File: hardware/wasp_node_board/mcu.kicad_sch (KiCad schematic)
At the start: 33 parts, among them J6 TC2030, SW2 C&K KMR231NG LFS, U1 STM32H723ZGTx, U3 APS6404L-3SQRx-SN, Y2 ASE-25.000MHZ-L-K-T

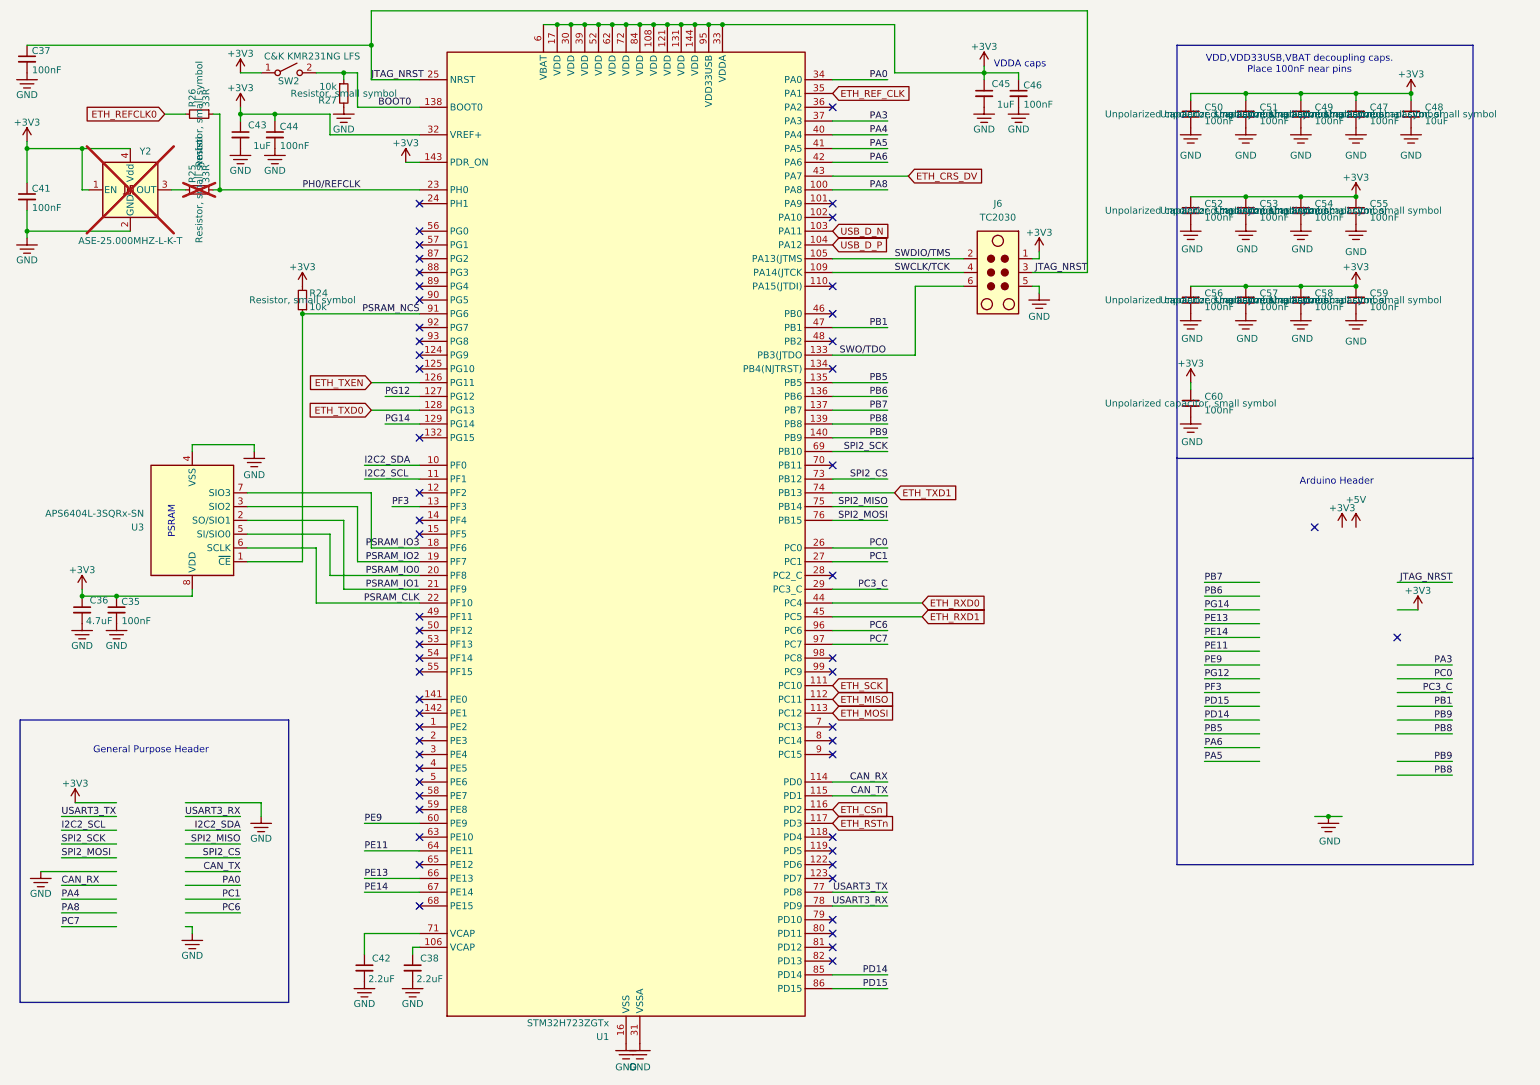
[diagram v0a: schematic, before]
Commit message: V1 layout done
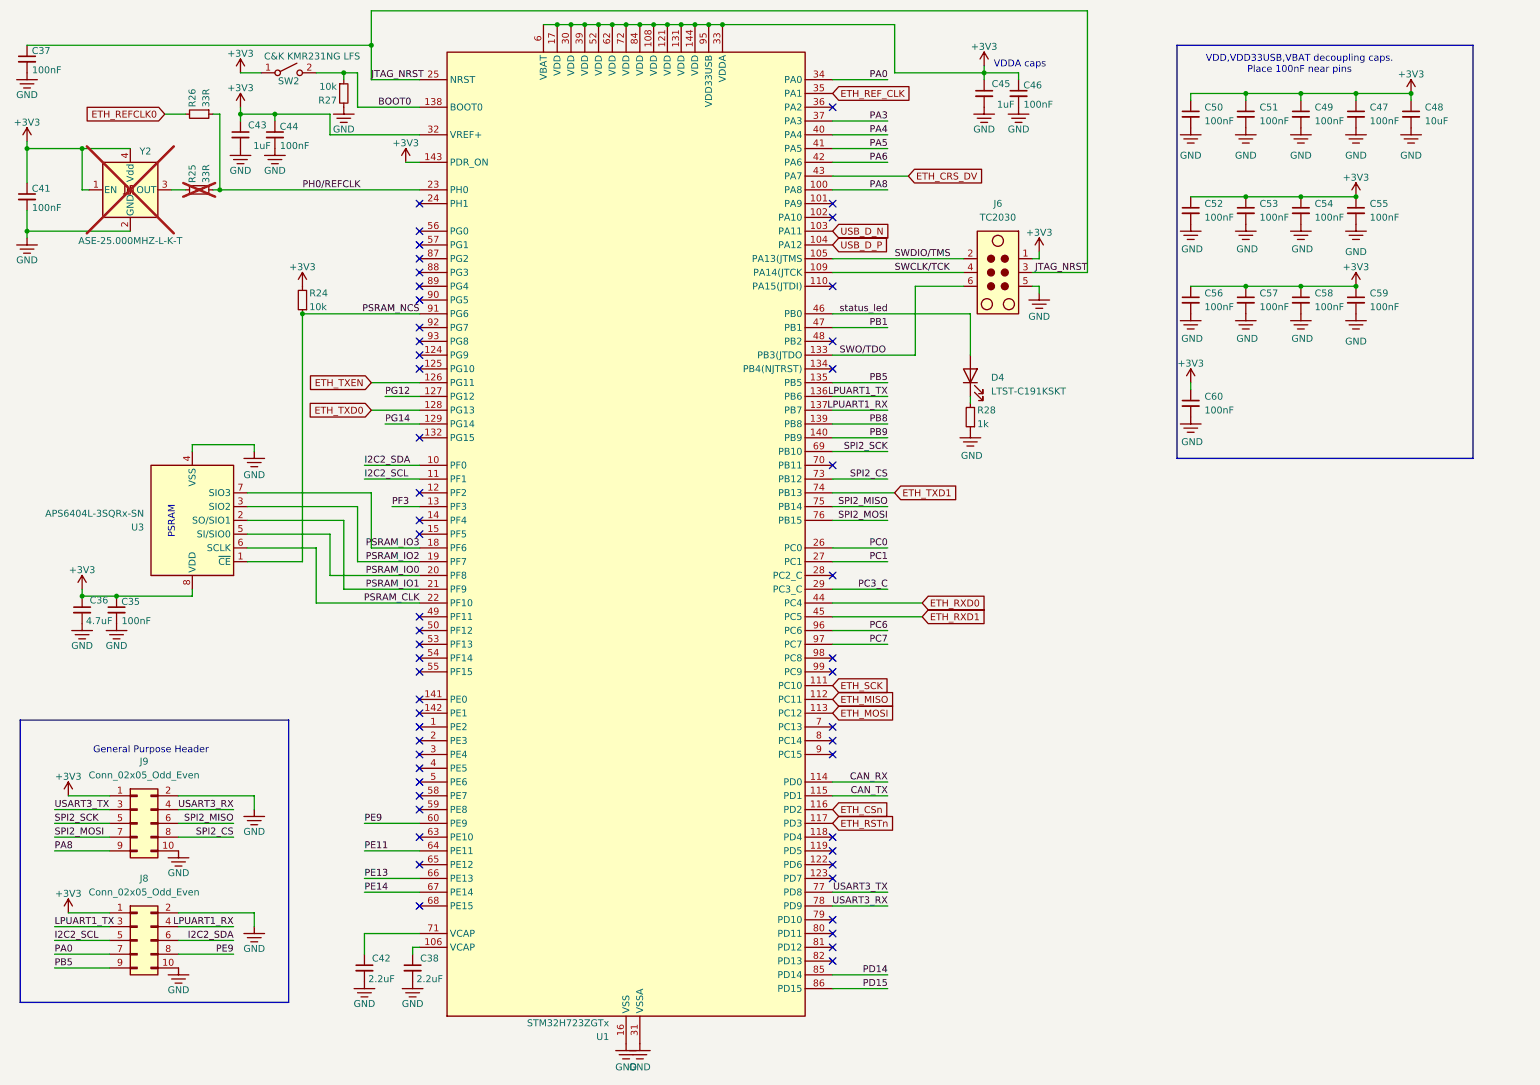
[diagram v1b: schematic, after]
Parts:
- added D4: LTST-C191KSKT, LED_SMD:LED_0603_1608Metric, symbol Device:LED
- added J8, J9: Conn_02x05_Odd_Even, Connector_PinHeader_2.54mm:PinHeader_2x05_P2.54mm_Vertical_SMD, symbol Connector_Generic:Conn_02x05_Odd_Even
- added R28: 1k, Resistor_SMD:R_0402_1005Metric, symbol Device:R_Small
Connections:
- net +3V3: now also J8.1 (Pin_1), J9.1 (Pin_1)
- net GND: now also J8.10 (Pin_10), J8.2 (Pin_2), J9.10 (Pin_10), J9.2 (Pin_2), R28.1
- net I2C2_SCL: now also J8.5 (Pin_5)
- net I2C2_SDA: now also J8.6 (Pin_6)
- net PA0: now also J8.7 (Pin_7)
- net PA8: now also J9.9 (Pin_9)
- net PB5: now also J8.9 (Pin_9)
- net PE9: now also J8.8 (Pin_8)
- net SPI2_CS: now also J9.8 (Pin_8)
- net SPI2_MISO: now also J9.6 (Pin_6)
- net SPI2_MOSI: now also J9.7 (Pin_7)
- net SPI2_SCK: now also J9.5 (Pin_5)
- net USART3_RX: now also J9.4 (Pin_4)
- net USART3_TX: now also J9.3 (Pin_3)
- net status_led: now reaches U1.46 (PB0)
- net status_led: now also D4.2 (A)
- net PB6 renamed LPUART1_TX
- net LPUART1_TX: now also J8.3 (Pin_3)
- net PB7 renamed LPUART1_RX
- net LPUART1_RX: now also J8.4 (Pin_4)
- new net: D4.1 (K), R28.2
- no-connect marks 56 -> 53
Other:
- note removed: "Arduino Header"
